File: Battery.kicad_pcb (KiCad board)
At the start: 2 copper layers, 57.4 x 58.3 mm, 9 parts, among them J1 USB_A

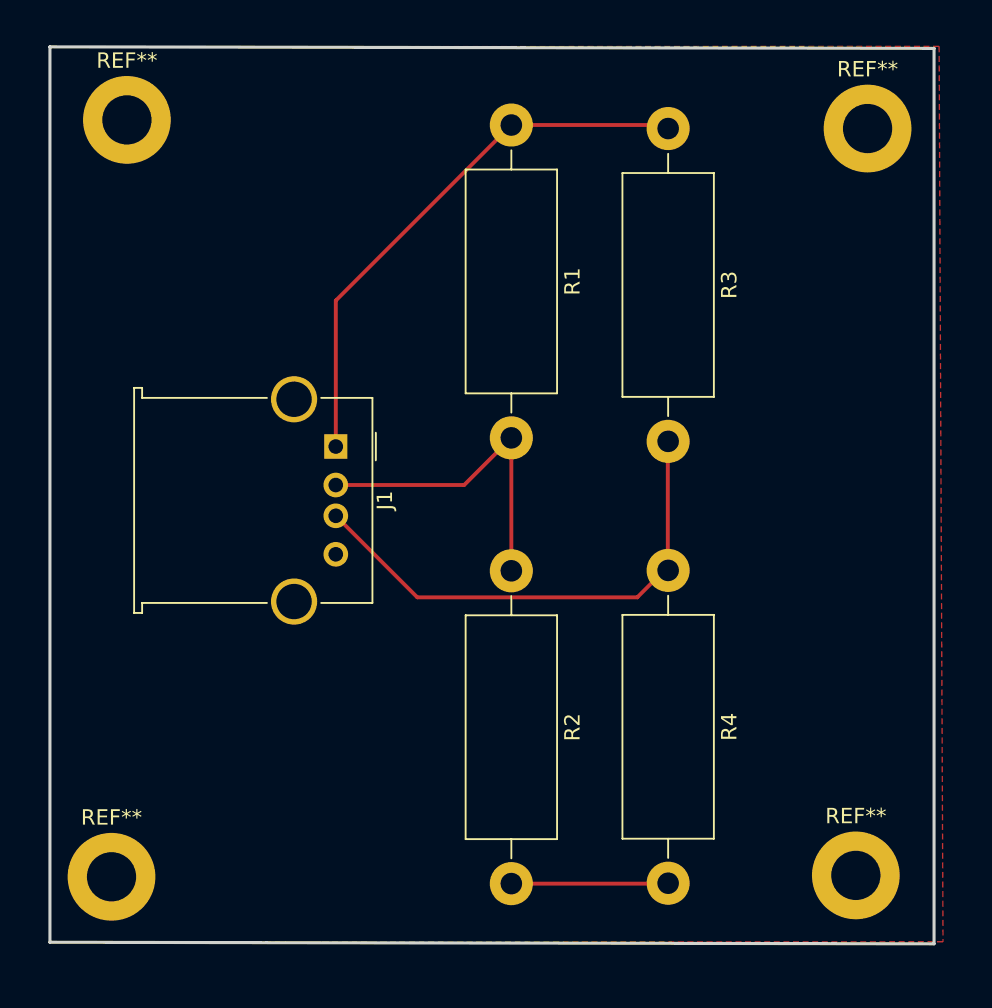
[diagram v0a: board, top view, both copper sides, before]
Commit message: up
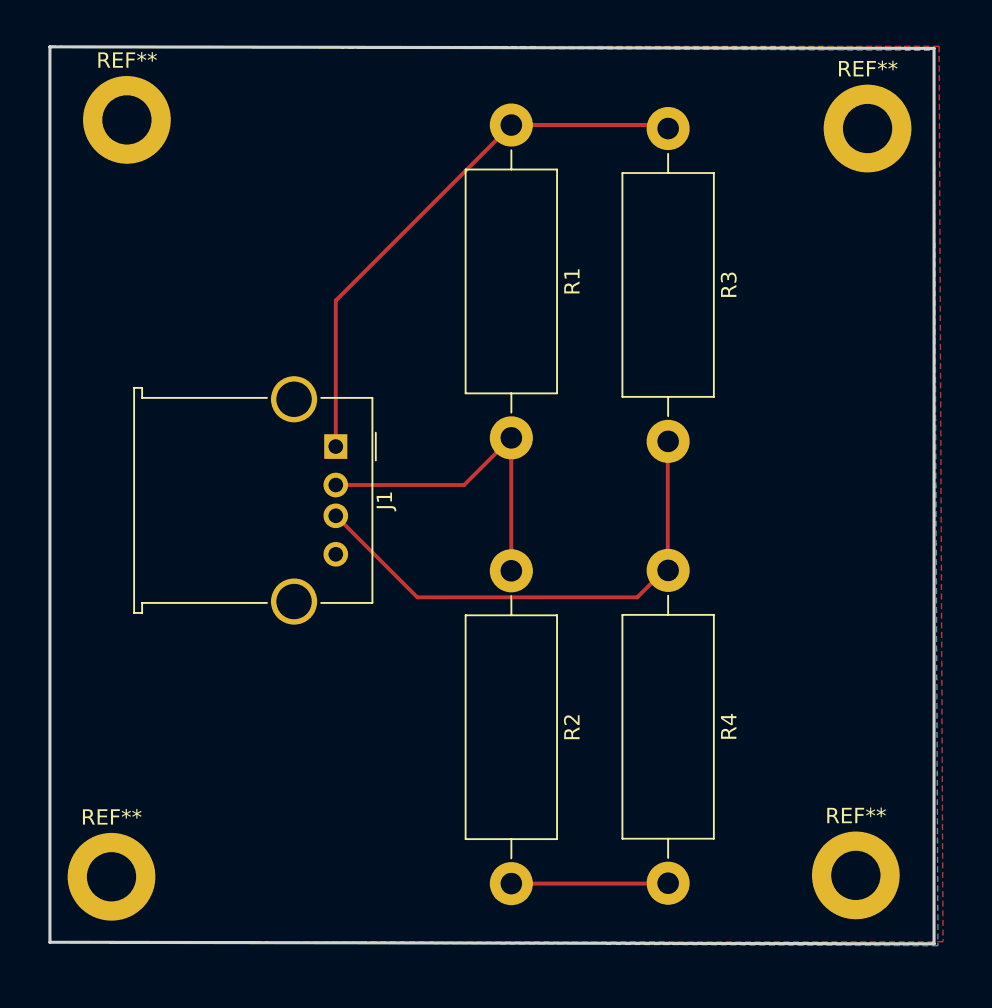
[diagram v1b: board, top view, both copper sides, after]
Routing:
- net +5VP: track 35.8 -> 46.0 mm
- added copper zone on B.Cu, net GND
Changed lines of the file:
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@@
       (effects (font (size 1 1) (thickness 0.15)))
     )
-    (fp_text value "MountingHole_3.2mm_M3_ISO7380_Pad" (at 0 3.85) (layer "F.Fab")
+    (fp_text value "MountingHole_3.2mm_M3_ISO7380_Pad" (at 10.758 -8.472) (layer "F.Fab")
       (effects (font (size 1 1) (thickness 0.15)))
     )
@@
   (gr_line (start 151.892 112.649) (end 94.462 112.548) (layer "Edge.Cuts") (width 0.2))
   (gr_line (start 94.462 54.382) (end 151.892 54.483) (layer "Edge.Cuts") (width 0.2))
+  (segment (start 113.03 80.346) (end 113.03 70.866) (width 0.25) (layer "F.Cu") (net 1))
+  (segment (start 124.434 59.462) (end 134.392 59.462) (width 0.25) (layer "F.Cu") (net 1))
+  (segment (start 124.434 59.462) (end 134.594 59.462) (width 0.25) (layer "F.Cu") (net 1))
+  (segment (start 134.392 59.462) (end 134.62 59.69) (width 0.25) (layer "F.Cu") (net 1))
   (segment (start 113.03 70.866) (end 124.434 59.462) (width 0.25) (layer "F.Cu") (net 1))
-  (segment (start 124.434 59.462) (end 134.594 59.462) (width 0.25) (layer "F.Cu") (net 1))
-  (segment (start 113.03 80.346) (end 113.03 70.866) (width 0.25) (layer "F.Cu") (net 1))
   (segment (start 113.03 82.846) (end 121.37 82.846) (width 0.25) (layer "F.Cu") (net 2))
   (segment (start 124.434 88.418) (end 124.434 79.782) (width 0.25) (layer "F.Cu") (net 2))
@@
       )
     )
+  )
+  (zone (net 4) (net_name "GND") (layer "B.Cu") (hatch edge 0.508)
+    (connect_pads (clearance 0.508))
+    (min_thickness 0.254) (filled_areas_thickness no)
+    (fill yes (thermal_gap 0.508) (thermal_bridge_width 0.508))
+    (polygon
+      (pts
+        (xy 151.892 54.61)
+        (xy 152.146 112.776)
+        (xy 94.488 112.522)
+        (xy 94.488 54.356)
+      )
+    )

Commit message: up
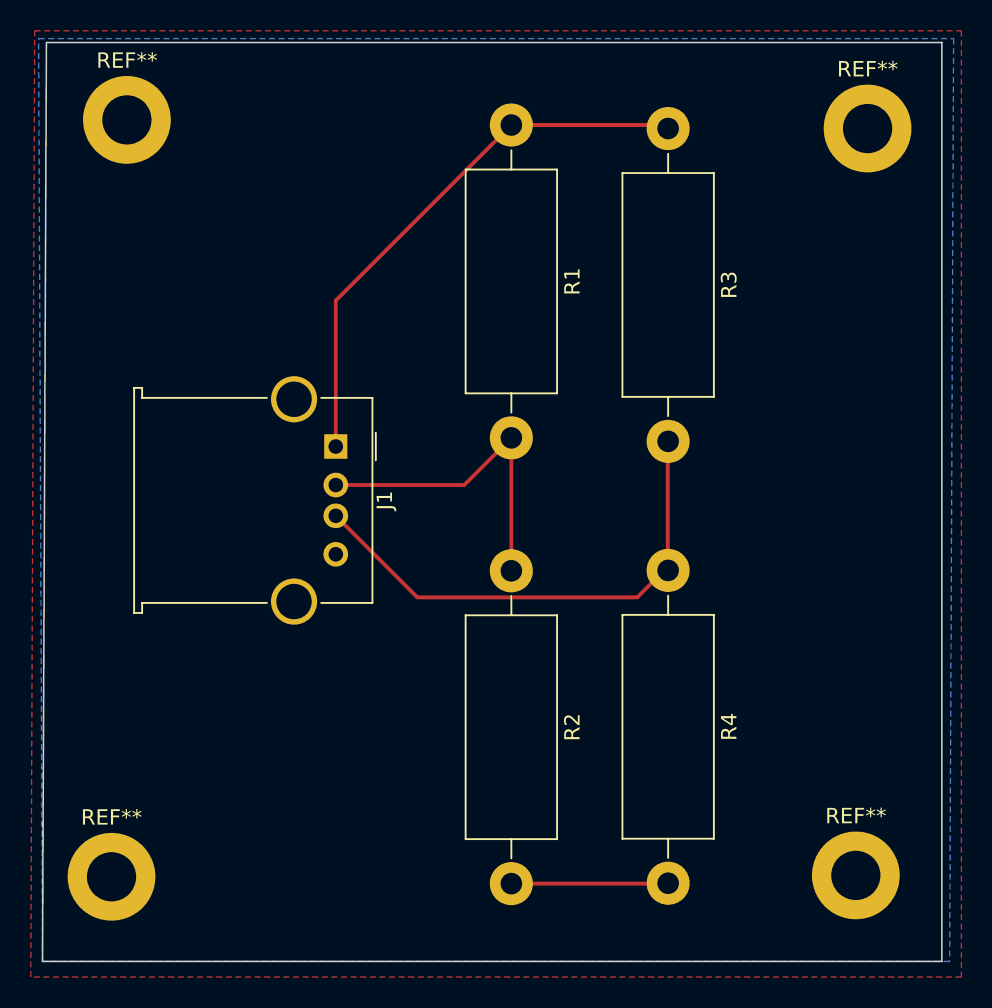
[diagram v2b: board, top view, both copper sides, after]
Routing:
- added copper zone on F.Cu, net +5VP
- removed copper zone on F.Cu, net GND
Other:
- board size 57.4 x 58.3 mm -> 58.4 x 59.7 mm
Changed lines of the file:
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@@
     (pad "1" thru_hole circle (at 0 0) (size 5.7 5.7) (drill 3.2) (layers *.Cu *.Mask))
   )
-  (gr_line (start 94.462 112.548) (end 94.462 54.382) (layer "Edge.Cuts") (width 0.2))
-  (gr_line (start 151.892 54.483) (end 151.892 112.649) (layer "Edge.Cuts") (width 0.2))
-  (gr_line (start 151.892 112.649) (end 94.462 112.548) (layer "Edge.Cuts") (width 0.2))
-  (gr_line (start 94.462 54.382) (end 151.892 54.483) (layer "Edge.Cuts") (width 0.2))
+  (gr_line (start 152.4 54.102) (end 152.4 113.792) (layer "Edge.Cuts") (width 0.1))
+  (gr_line (start 93.98 113.792) (end 94.234 54.102) (layer "Edge.Cuts") (width 0.1))
+  (gr_line (start 94.234 54.102) (end 152.4 54.102) (layer "Edge.Cuts") (width 0.1))
+  (gr_line (start 152.4 113.792) (end 93.98 113.792) (layer "Edge.Cuts") (width 0.1))
   (segment (start 113.03 80.346) (end 113.03 70.866) (width 0.25) (layer "F.Cu") (net 1))
   (segment (start 124.434 59.462) (end 134.392 59.462) (width 0.25) (layer "F.Cu") (net 1))
@@
   (segment (start 118.327 90.143) (end 132.615 90.143) (width 0.25) (layer "F.Cu") (net 3))
   (segment (start 124.434 108.738) (end 134.594 108.738) (width 0.25) (layer "F.Cu") (net 4))
-  (zone (net 4) (net_name "GND") (layer "F.Cu") (hatch edge 0.508)
+  (zone (net 1) (net_name "+5VP") (layer "F.Cu") (hatch edge 0.508)
     (connect_pads (clearance 0.508))
     (min_thickness 0.254) (filled_areas_thickness no)
@@
     (polygon
       (pts
-        (xy 152.474789 112.515394)
-        (xy 94.462 112.548)
-        (xy 94.462 54.382)
-        (xy 152.220789 54.349394)
+        (xy 153.67 114.808)
+        (xy 93.218 114.808)
+        (xy 93.472 53.34)
+        (xy 153.67 53.34)
       )
     )
@@
     (polygon
       (pts
-        (xy 151.892 54.61)
-        (xy 152.146 112.776)
-        (xy 94.488 112.522)
-        (xy 94.488 54.356)
+        (xy 153.162 53.848)
+        (xy 152.908 113.792)
+        (xy 93.98 113.792)
+        (xy 93.726 53.848)
       )
     )
